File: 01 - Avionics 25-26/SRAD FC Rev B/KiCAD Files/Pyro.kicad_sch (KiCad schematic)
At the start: 22 parts, among them J2 282834-2, J3 282834-4, U2 ZXCT1110W5-7, U5 SI9926CDY

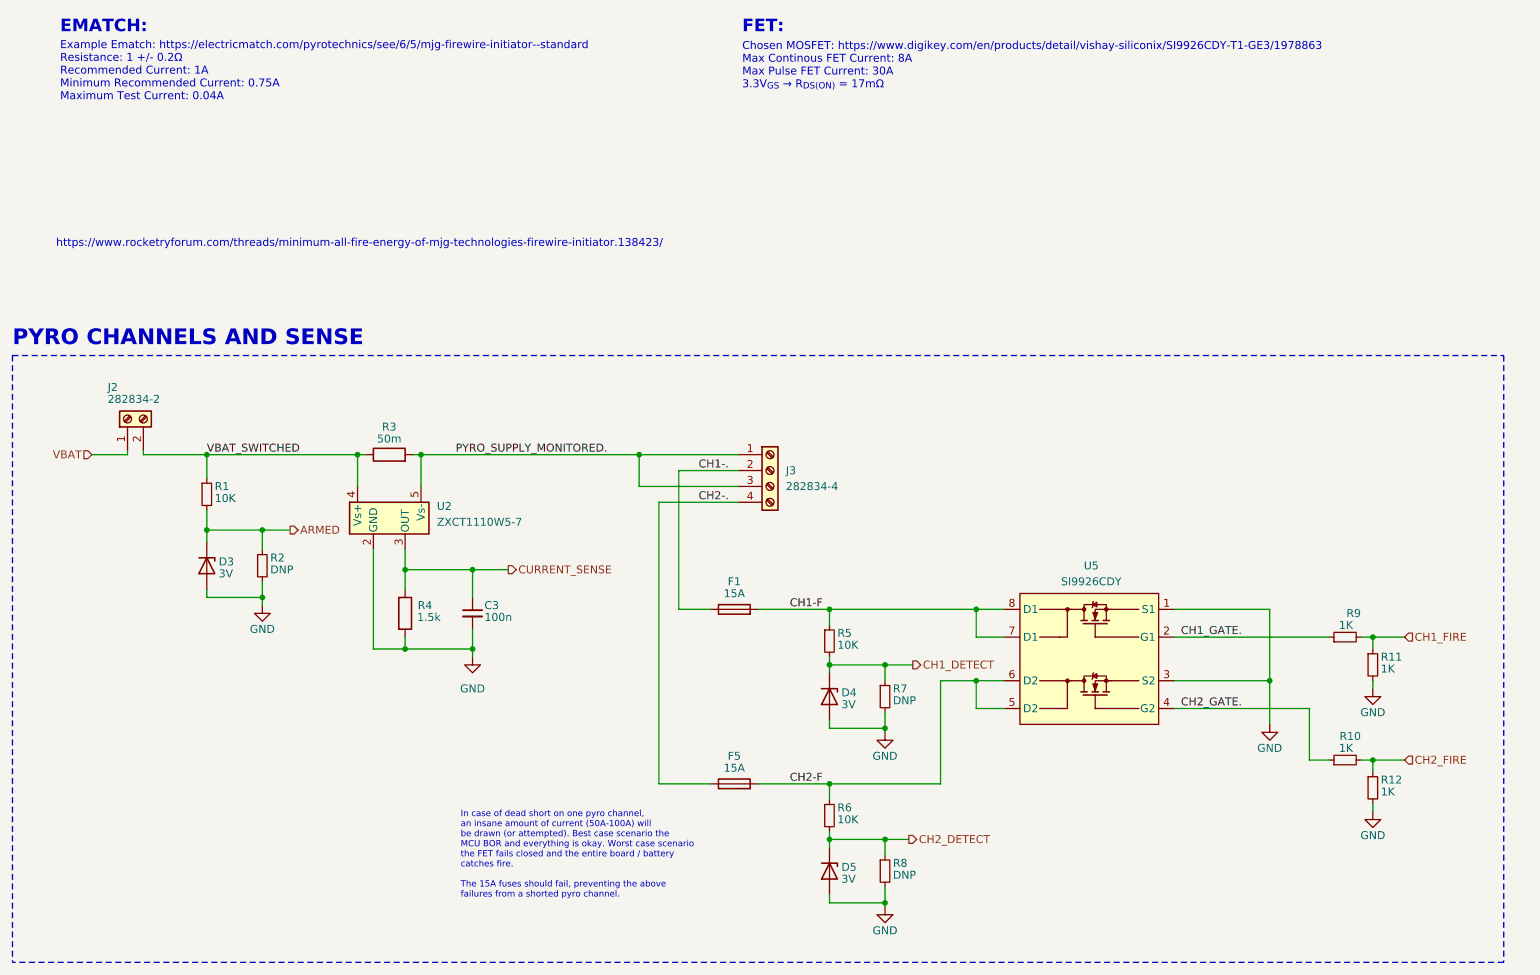
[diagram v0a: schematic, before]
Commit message: some fixes from seth's feedback
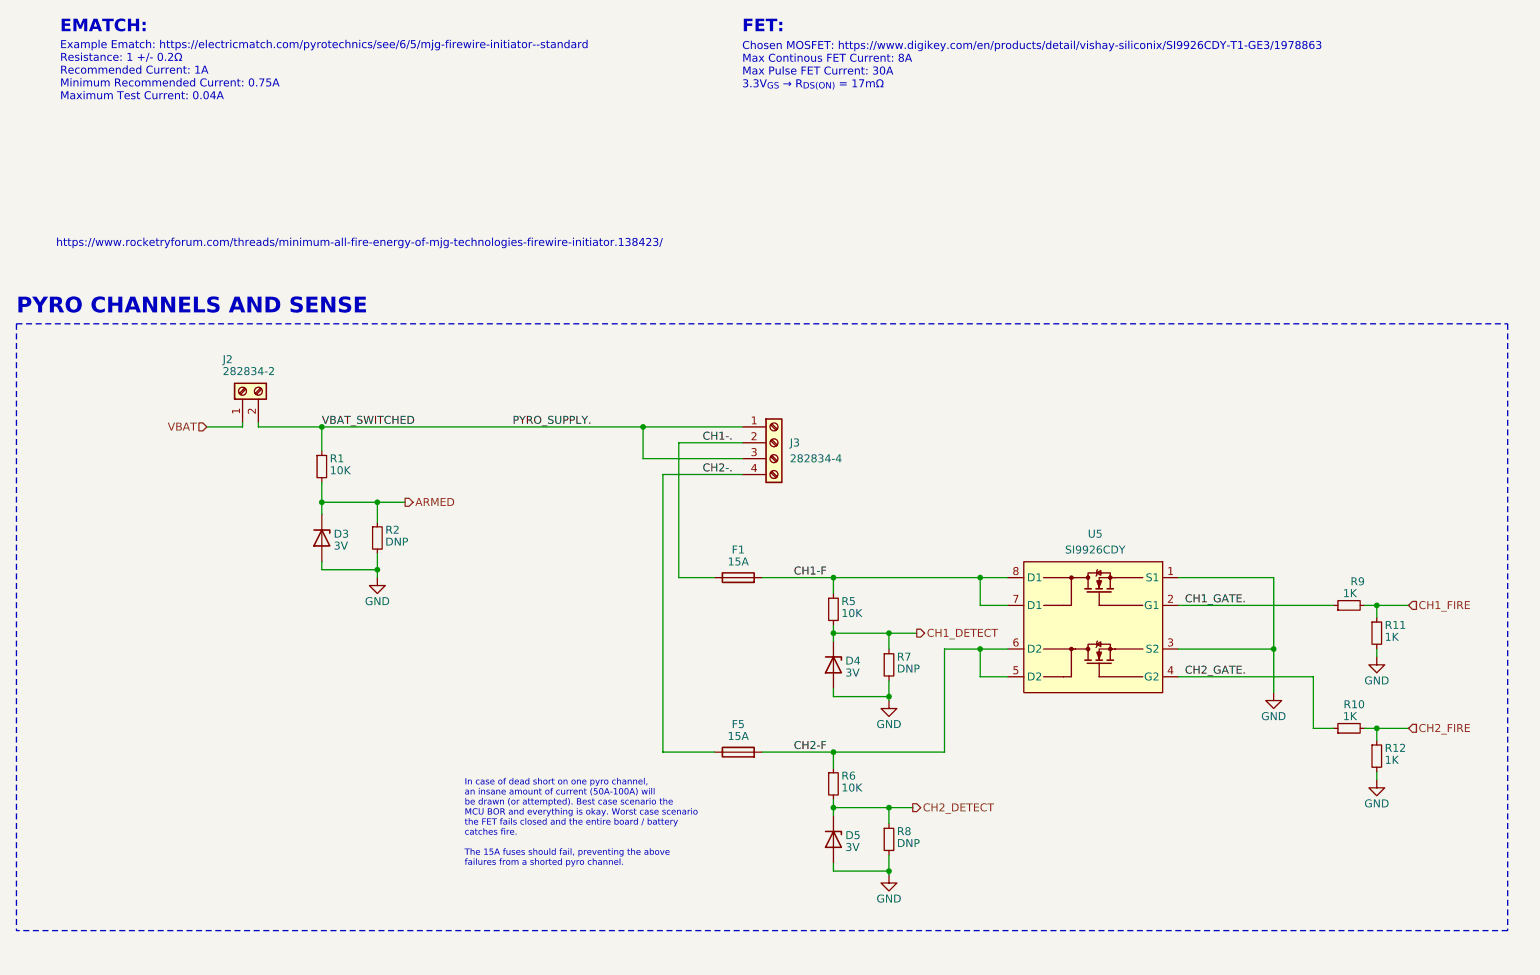
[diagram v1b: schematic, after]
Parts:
- removed C3: 100n, Resistor_SMD:R_0603_1608Metric, symbol Device:C_Small
- removed R3: 50m, Resistor_SMD:R_0603_1608Metric, symbol Device:R
- removed R4: 1.5k, Resistor_SMD:R_0603_1608Metric, symbol Device:R
- removed U2: ZXCT1110W5-7, Package_TO_SOT_SMD:SOT-23-5, symbol Amplifier_Current:ZXCT1110
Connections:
- net VBAT_SWITCHED is gone; now on net PYRO_SUPPLY.: J2.2 (Pin_2), R1.1
- net PYRO_SUPPLY_MONITORED. renamed PYRO_SUPPLY.
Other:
- moved on the sheet: D3, D4, D5, F1, F5, J2, J3, R1, R10, R11, R12, R2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
